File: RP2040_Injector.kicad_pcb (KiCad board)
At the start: 2 copper layers, 63.9 x 14 mm, 25 parts, among them J1 USB-A, J2 Conn_01x02, U1 NCP1117-3.3_SOT223, U2 W25Q128JVS, U3 RP2040

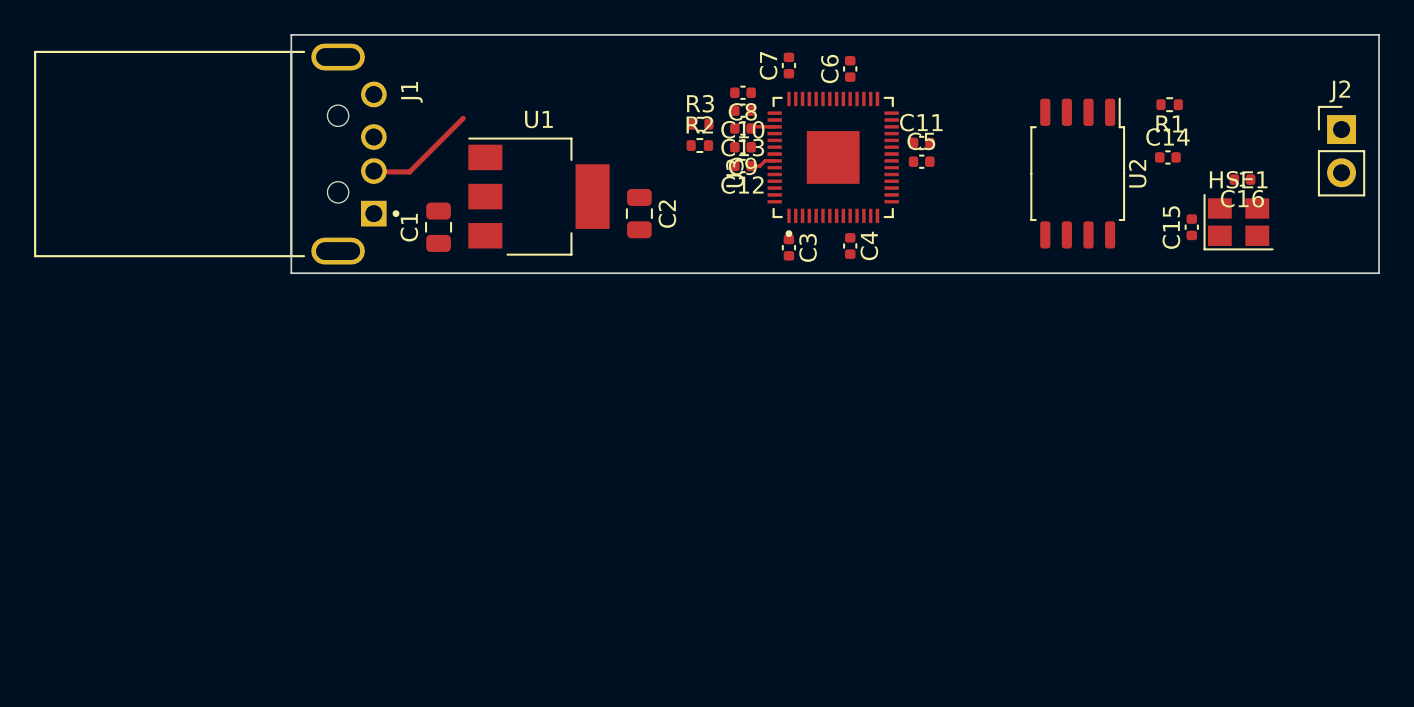
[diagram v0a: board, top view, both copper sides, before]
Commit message: Finished v0.1 PCB wiring
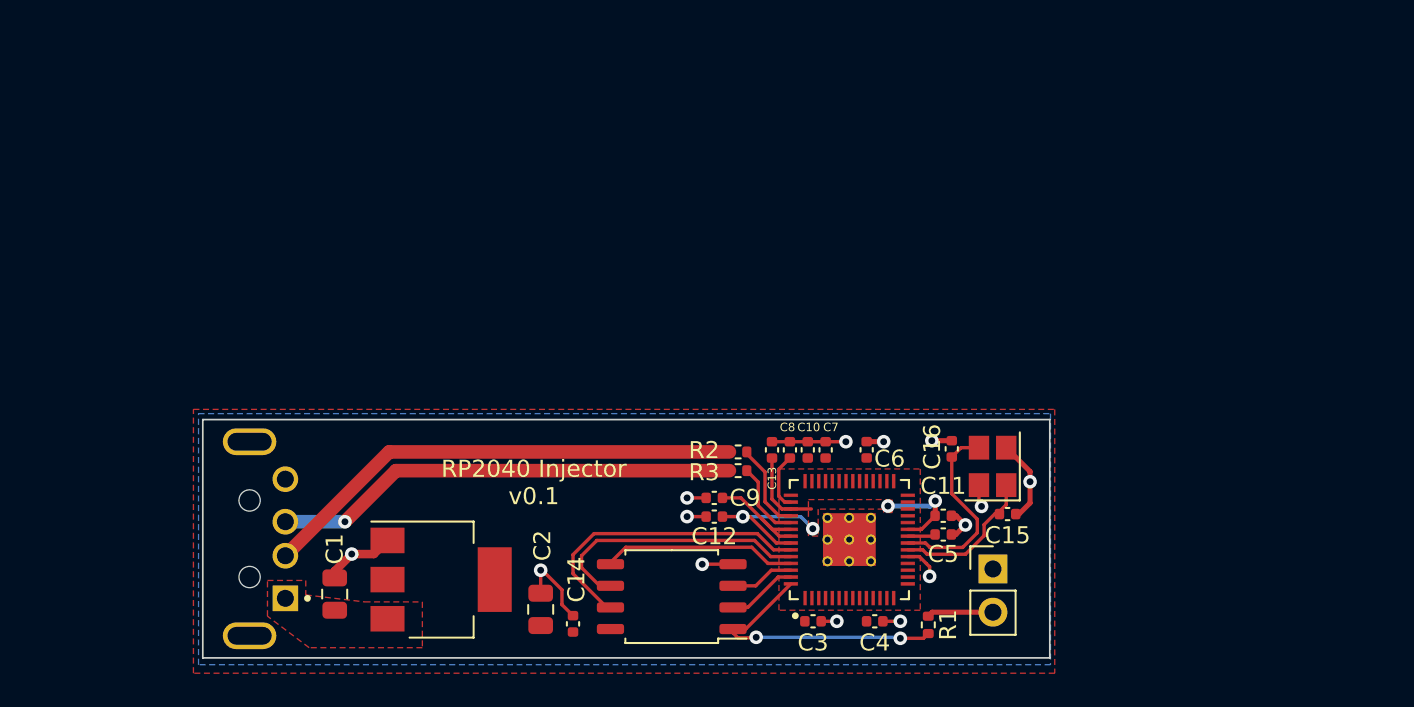
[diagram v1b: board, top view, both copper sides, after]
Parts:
- added ?: , , F.Cu at (163.8, 99.9)
- added ?: , , F.Cu at (161.2, 99.9)
- added ?: , , F.Cu at (162.5, 101.2)
- added ?: , , F.Cu at (163.8, 101.2)
- added ?: , , F.Cu at (162.5, 102.4)
- added ?: , , F.Cu at (161.2, 102.4)
- added ?: , , F.Cu at (162.5, 99.9)
- added ?: , , F.Cu at (163.8, 102.4)
- added ?: , , F.Cu at (161.2, 101.2)
- moved C14 44.4 mm to (146.3, 106.1), turned to 90 degrees
- moved U2 34.4 mm to (152.1, 104.5), turned to 180 degrees
- moved R1 33.7 mm to (167.2, 106.2), turned to -90 degrees
- moved J2 33.0 mm to (171.0, 102.9)
- moved C2 24.0 mm to (144.4, 105.2), turned to 90 degrees
- moved C16 23.3 mm to (168.6, 95.8), turned to 90 degrees
- moved U1 23.2 mm to (138.6, 103.5)
- moved J1 23.2 mm to (127.3, 101.1)
- moved C7 22.7 mm to (161.1, 95.9)
- moved U3 22.5 mm to (162.5, 101.2)
- moved C1 22.4 mm to (132.3, 104.3)
- moved C6 22.4 mm to (163.6, 95.9)
- moved C4 22.1 mm to (164.0, 106.0), turned to 0 degrees
- moved C3 22.0 mm to (160.4, 106.0), turned to 0 degrees
- moved C11 21.9 mm to (168.1, 99.8)
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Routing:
- net GND: track 0.00 -> 32.1 mm, vias 0 -> 14
- net USB_DP: track 0.00 -> 27.3 mm, vias 0 -> 1
- net USB_DM: track 6.20 -> 28.6 mm
- net /QSPI_SD3: track 0.00 -> 17.8 mm
- net +1V1: track 2.94 -> 19.9 mm, vias 0 -> 4
- net /QSPI_CSN: track 0.00 -> 16.5 mm, vias 0 -> 2
- net /QSPI_SCLK: track 0.00 -> 15.9 mm
- net +3V3: track 0.00 -> 11.9 mm
- net /QSPI_SD0: track 0.00 -> 11.5 mm
- net XOUT: track 0.00 -> 11.4 mm
- net XIN: track 0.00 -> 8.71 mm
- net Net-(R2-Pad2): track 0.00 -> 5.23 mm
- net Net-(R3-Pad2): track 0.00 -> 4.66 mm
- net /QSPI_SD1: track 0.00 -> 4.14 mm
- net /~{USB_BOOT}: track 0.00 -> 3.90 mm
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- added copper zone on F.Cu, net +1V1
- added copper zone on F.Cu, net +3V3
- added copper zone on B.Cu, net GND
- added copper zone on F.Cu, net VCC
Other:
- board size 63.9 x 14 mm -> 49.8 x 14 mm
- board text added: "BSC 8/22"
- board text added: "RP2040 Injector v0.1"
